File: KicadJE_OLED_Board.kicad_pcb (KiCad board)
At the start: 2 copper layers, 170.6 x 128 mm, 296 parts, among them J1 LED 1-6, J101 Out1, J102 IN1, J103 OUT1, J104 OutFlt, J105 INFLT, J106 OUTFLT, J107 In1_Flt, J108 InAmp, J201 OLED, J202 ADC Input, J203 Out2, J204 Out1, J205 OUT1, J206 OUT2, J207 IN1, J208 IN2, J209 CV1, J210 CV2, J211 FrontLED, J212 -12V Front, J301 UART, J302 AVR-ISP-6, J401 Out2, J402 Out1, J403 OUT1, J404 OUT2, J405 IN1, J406 IN2, J407 CV1, J408 CV2, J409 -12V Front, J410 OLED, J411 ADC Input, J412 FrontLED, J501 UART, J502 AVR-ISP-6, P1 Doepfer_Power_16pin, P101 Doepfer_Power_10pin, P201 Doepfer_Power_16pin, P401 Doepfer_Power_16pin, SW201 Rotary_Encoder_Switch, SW202 Rotary_Encoder_Switch, SW401 Rotary_Encoder_Switch, SW402 Rotary_Encoder_Switch, U101 TL072, U201 TL072, U202 TL072, U301 ATmega32A-AU, U401 TL072, U402 MCP4822, U501 ATmega32A-AU, Y301 16MHz, Y501 16MHz

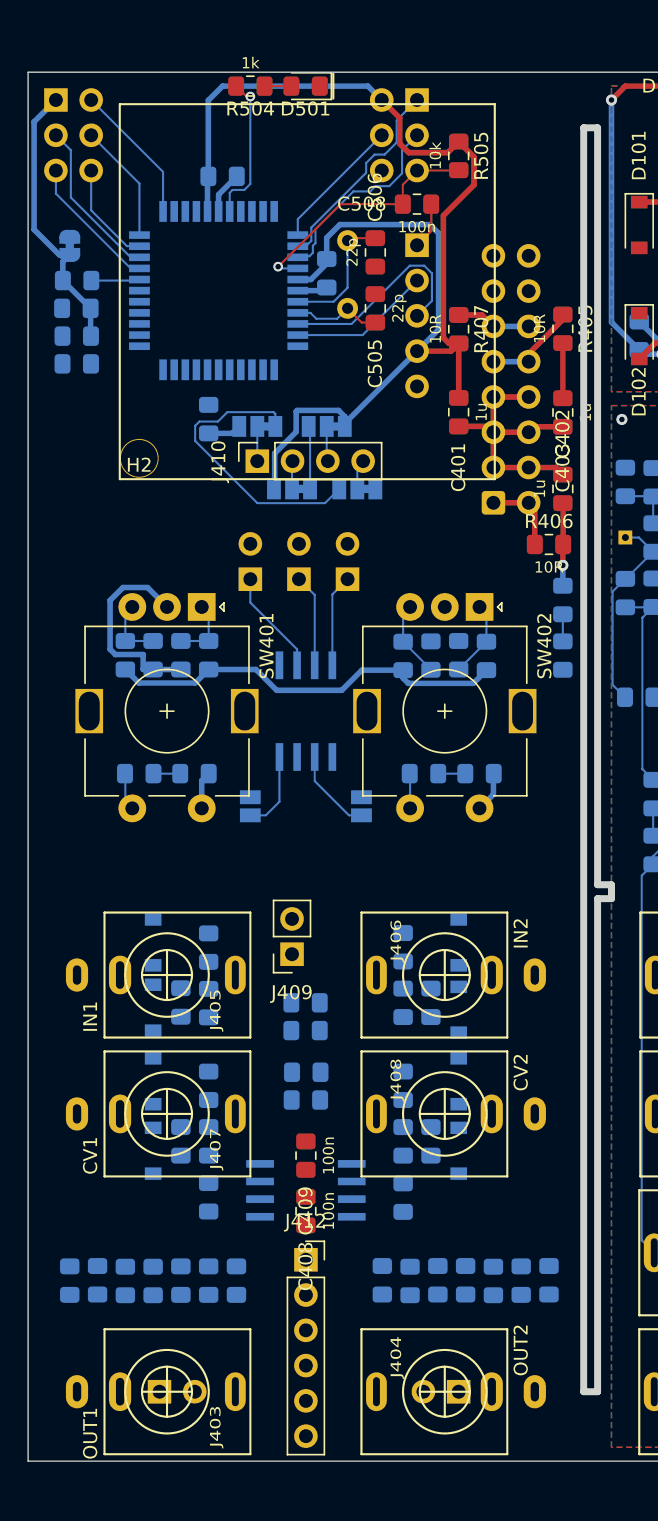
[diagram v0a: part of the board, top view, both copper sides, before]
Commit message: Initial DAC layout
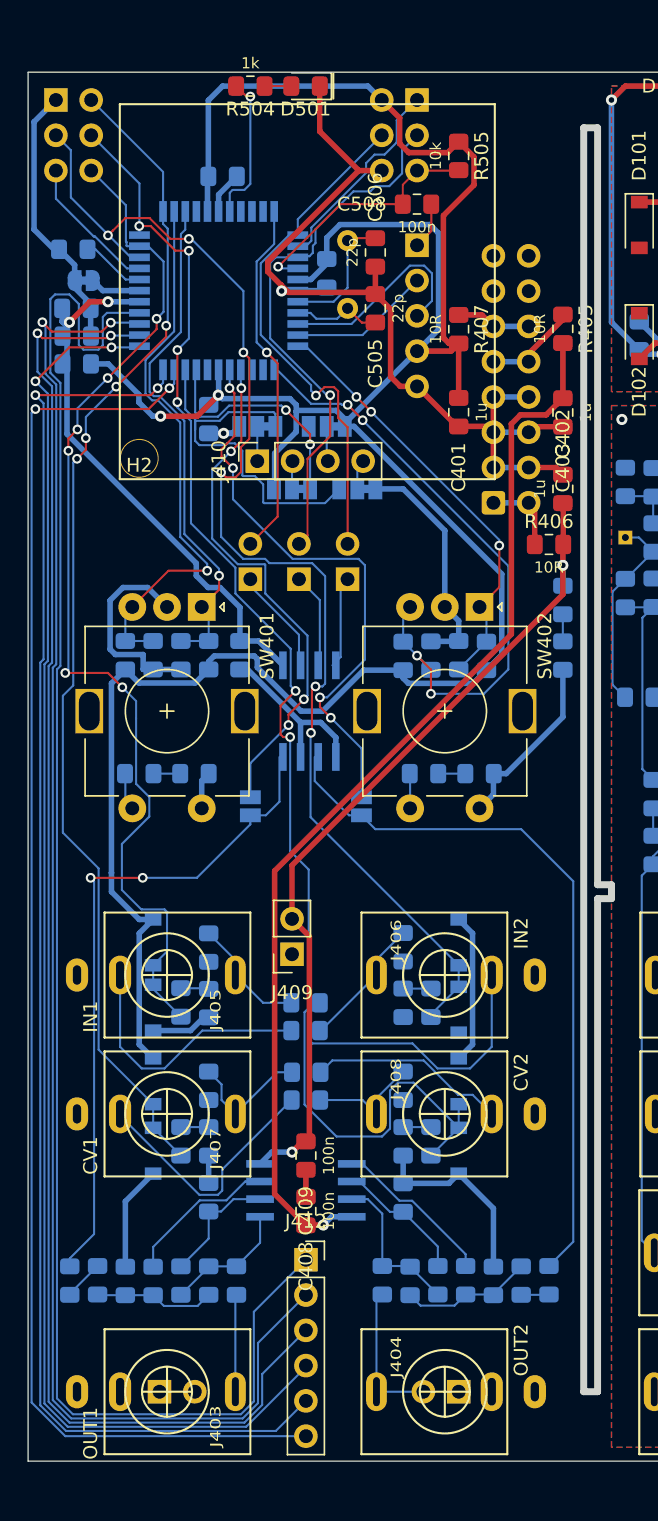
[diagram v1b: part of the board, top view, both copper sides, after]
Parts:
- added C422: 100n, AJ:C_0805_AJ, B.Cu at (115.2, 92.0)
- moved R502 2.69 mm to (104.0, 65.0), turned to 0 degrees
- moved C507 2.27 mm to (103.2, 62.8)
- moved U402 0.25 mm to (120.2, 96.0)
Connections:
- J502 pad 3: /KicadJE_ATMega32A_DAC/sheet6241082B/D7_SCK -> SCK_DAC
- J502 pad 4: /KicadJE_ATMega32A_DAC/sheet6241082B/D5_MOSI -> MOSI_DAC
- JP407 pad 2: Net-(JP407-Pad2) -> CS_DAC
- JP408 pad 2: Net-(JP408-Pad2) -> MOSI_DAC
- JP409 pad 2: Net-(JP409-Pad2) -> SCK_DAC
- U501 pad 1: /KicadJE_ATMega32A_DAC/sheet6241082B/D5_MOSI -> MOSI_DAC
- U501 pad 3: /KicadJE_ATMega32A_DAC/sheet6241082B/D7_SCK -> SCK_DAC
- U501 pad 44: /KicadJE_ATMega32A_DAC/sheet6241082B/D4 -> CS_DAC
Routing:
- net /KicadJE_ATMega32A_DAC/sheet6241082B/D23: track 0.00 -> 118.6 mm
- net /KicadJE_ATMega32A_DAC/sheet6241082B/D22: track 0.00 -> 110.7 mm, vias 0 -> 2
- net /KicadJE_ATMega32A_DAC/sheet6241082B/D21: track 0.00 -> 108.2 mm, vias 0 -> 2
- net /KicadJE_ATMega32A_DAC/sheet6241082B/D19: track 0.00 -> 104.3 mm, vias 0 -> 2
- net /KicadJE_ATMega32A_DAC/sheet6241082B/D18: track 0.00 -> 104.1 mm, vias 0 -> 2
- net /KicadJE_ATMega32A_DAC/sheet6241082B/D20: track 0.00 -> 104.0 mm, vias 0 -> 2
- net 28_A4_DAC: track 8.62 -> 101.1 mm, vias 0 -> 6
- net +5V: track 123.4 -> 211.9 mm, vias 0 -> 2
- net 30_A6_DAC: track 11.6 -> 90.3 mm, vias 0 -> 6
- net 27_A3_DAC: track 10.2 -> 84.9 mm, vias 0 -> 4
- net GND: track 71.9 -> 146.6 mm, vias 0 -> 2
- net +12V: track 3.97 -> 77.7 mm, vias 0 -> 1
- net 29_A5_DAC: track 7.41 -> 75.6 mm, vias 0 -> 6
- net -12V: track 5.97 -> 60.1 mm, vias 1 -> 2
- net DACB: track 6.12 -> 51.8 mm
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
